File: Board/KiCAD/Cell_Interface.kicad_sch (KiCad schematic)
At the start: 32 parts, among them Q23 2N7002, Q24 2N7002, Q25 2N7002, Q26 2N7002, Q27 IRF9540NSTRLPBF, Q28 IRF9540NSTRLPBF, Q29 IRF9540NSTRLPBF, Q30 IRF9540NSTRLPBF, Q31 IRF9540NSTRLPBF, Q32 2N7002, Q33 IRF9540NSTRLPBF, U4 INA260, U6 INA260, U7 INA260, U8 INA260

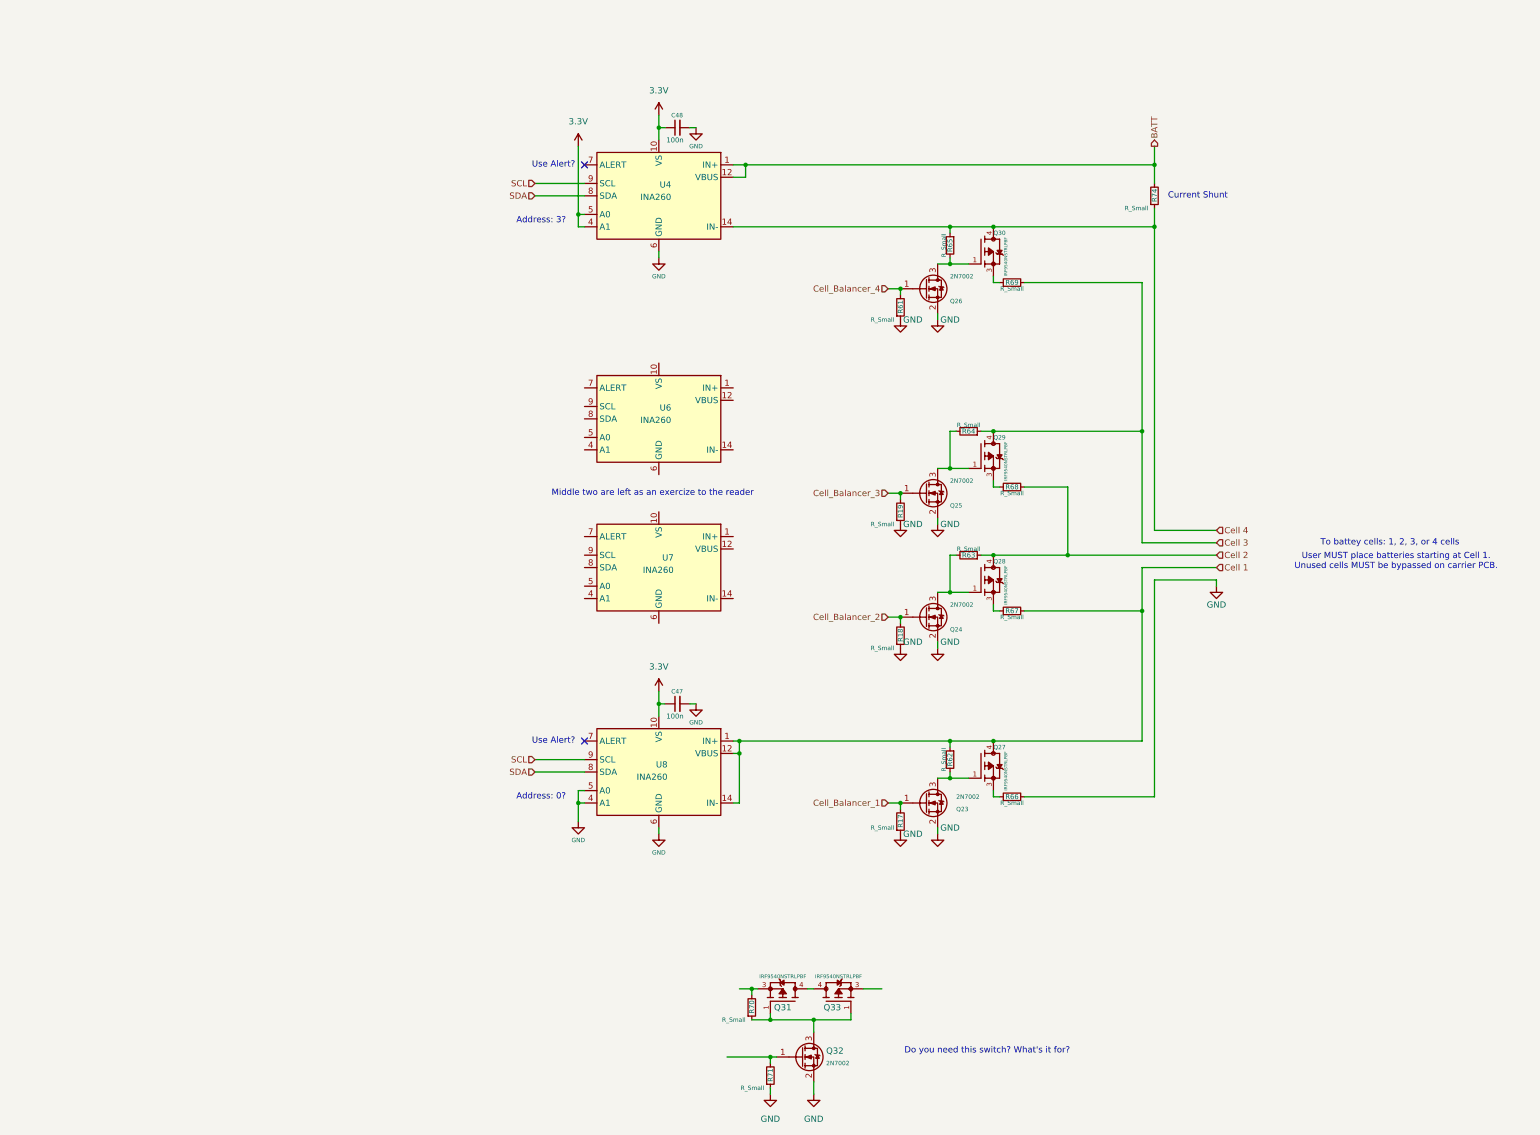
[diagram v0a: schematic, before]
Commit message: Add files via upload
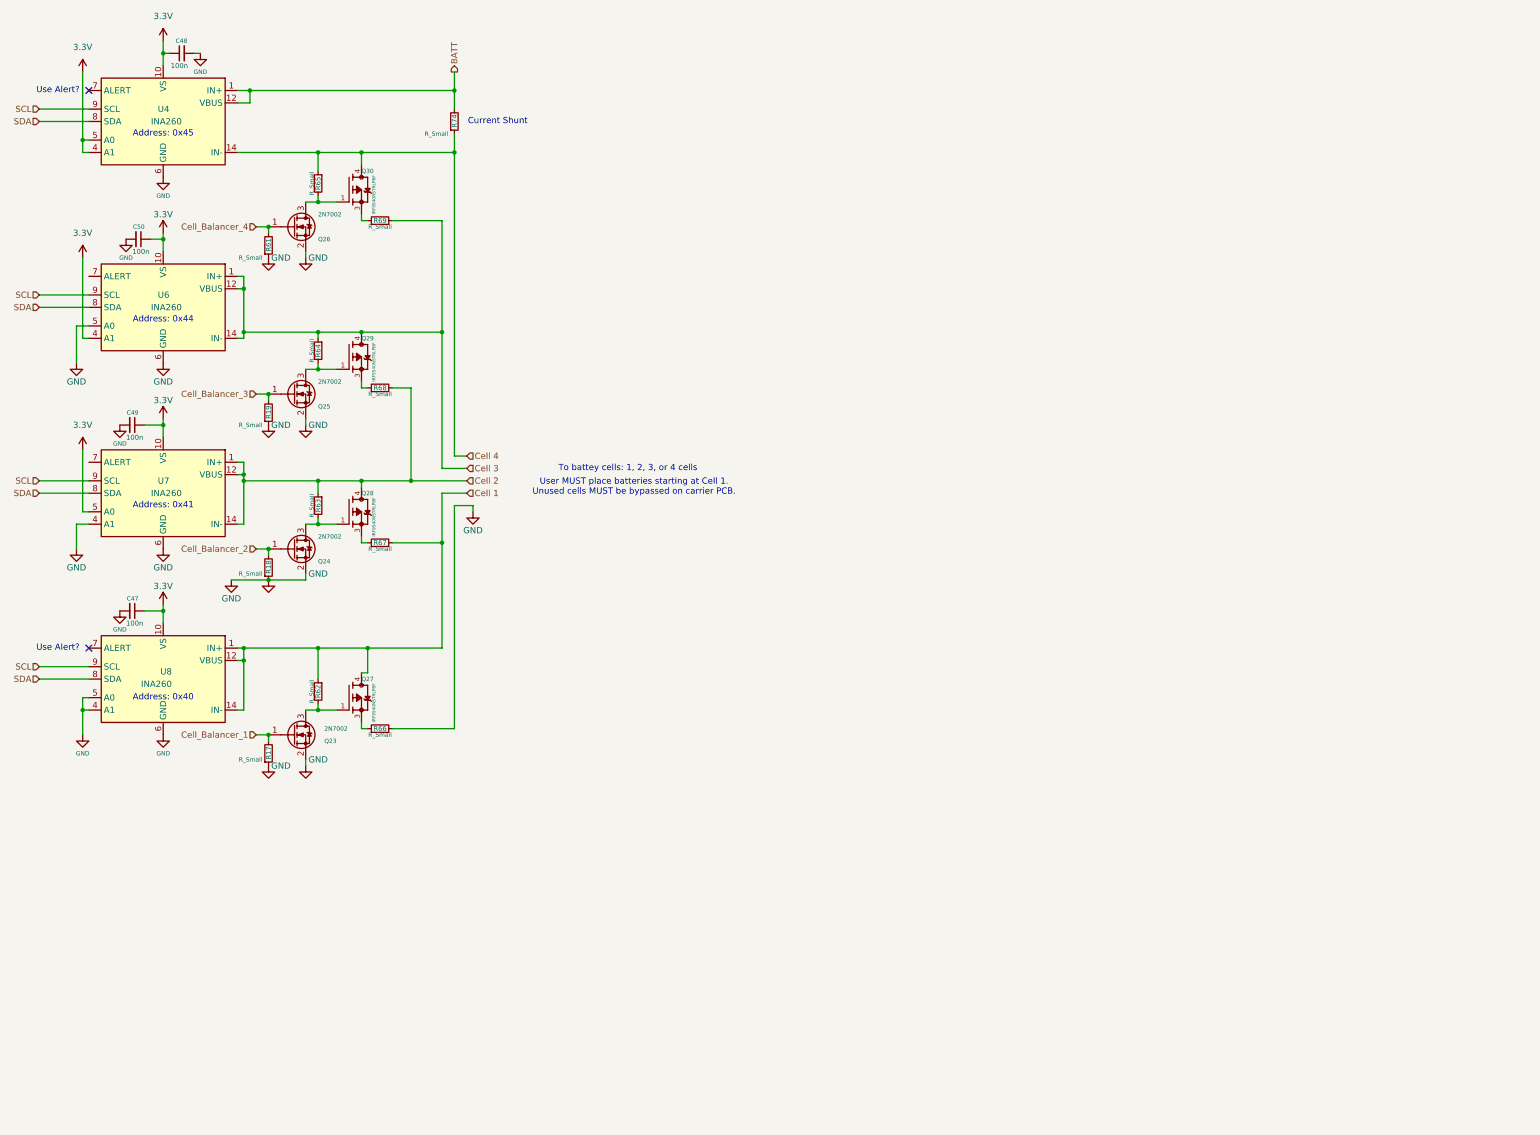
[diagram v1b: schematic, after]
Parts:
- removed Q31, Q33: IRF9540NSTRLPBF, IRF9540NSTRLPBF:DPAK254P1524X483-4_3N, symbol IRF9540NSTRLPBF:IRF9540NSTRLPBF
- removed Q32: 2N7002, Package_TO_SOT_SMD:SOT-23, symbol Transistor_FET:2N7002
- removed R70: R_Small, symbol Device:R_Small
- removed R71: R_Small, Resistor_SMD:R_0201_0603Metric, symbol Device:R_Small
- added C49, C50: 100n, Capacitor_SMD:C_0201_0603Metric, symbol Device:C_Small
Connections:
- net 3.3V: now also U6.10 (VS), U6.4 (A1), U7.10 (VS), U7.5 (A0), C49.1, C50.1
- net Cell 2: now also U7.1 (IN+), U7.12 (VBUS), U7.14 (IN-)
- net Cell 3: now also U6.1 (IN+), U6.12 (VBUS), U6.14 (IN-)
- net GND: now also U6.5 (A0), U6.6 (GND), U7.4 (A1), U7.6 (GND), C49.2, C50.2
- net SCL: now also U6.9 (SCL), U7.9 (SCL)
- net SDA: now also U6.8 (SDA), U7.8 (SDA)
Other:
- note added: "Address: 0x40"
- note added: "Address: 0x41"
- note added: "Address: 0x44"
- note added: "Address: 0x45"
- note removed: "Address: 0?"
- note removed: "Address: 3?"
- note removed: "Do you need this switch? What's it for?"
- note removed: "Middle two are left as an exercize to the reader"
- moved on the sheet: C47, C48, Q23, Q24, Q25, Q26, Q27, Q28, Q29, Q30, R17, R18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

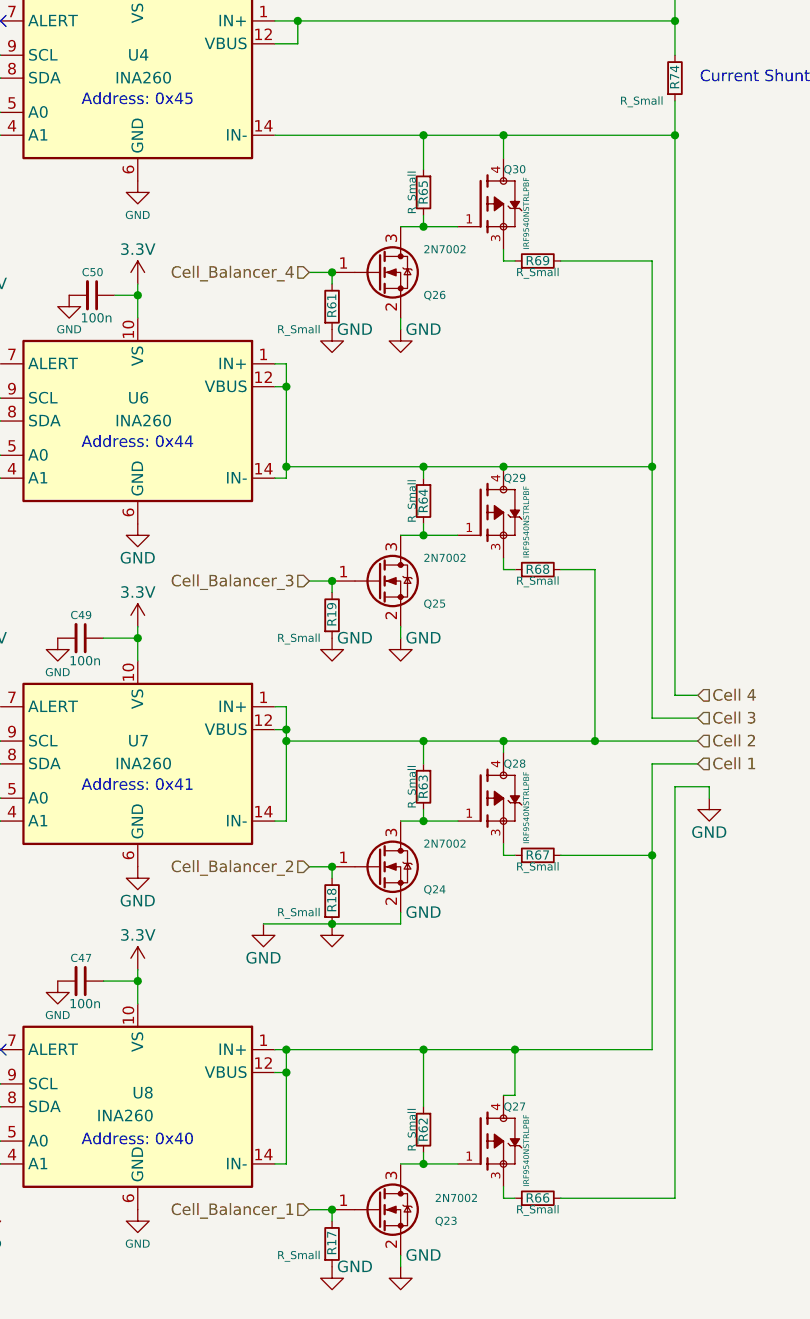
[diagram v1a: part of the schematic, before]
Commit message: Add files via upload
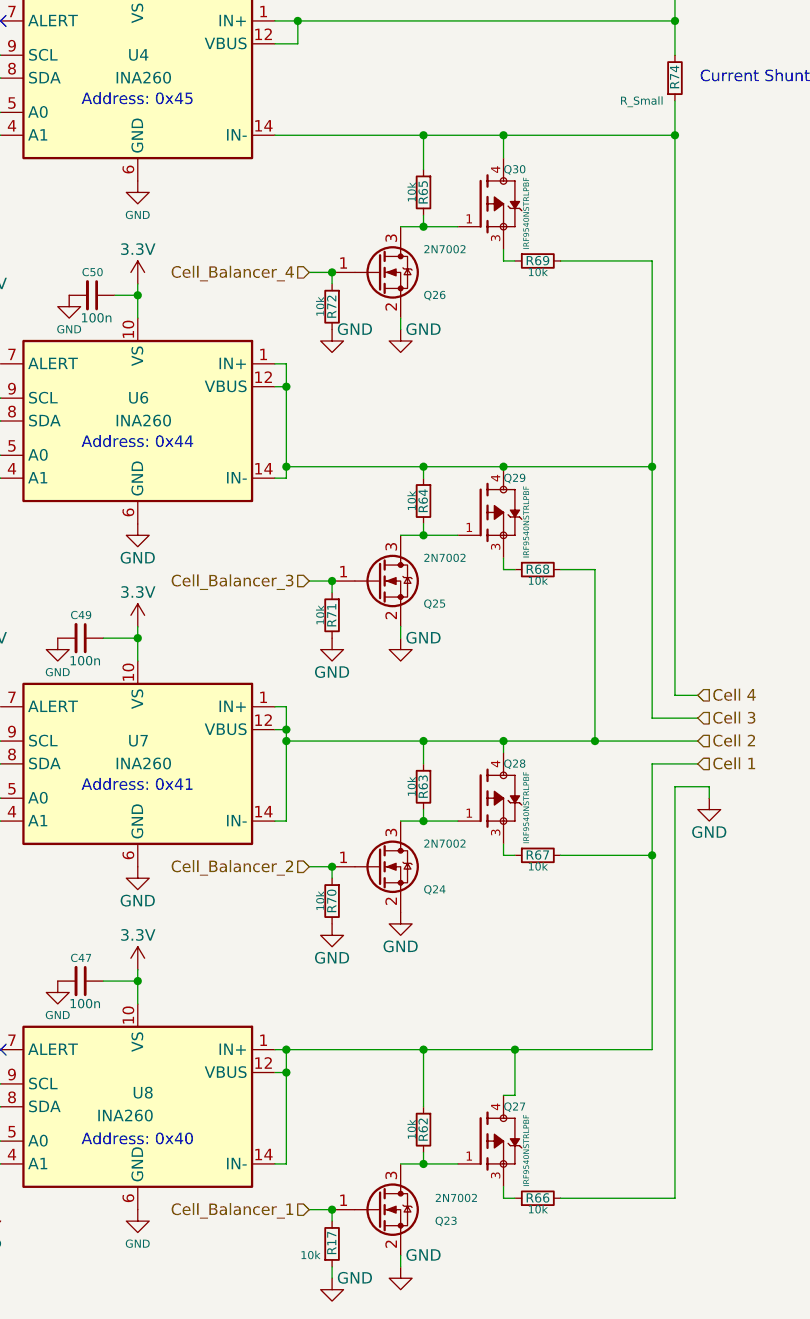
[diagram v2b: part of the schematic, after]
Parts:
- removed R18, R19, R61: R_Small, Resistor_SMD:R_0201_0603Metric, symbol Device:R_Small
- added R70, R71, R72: 10k, Resistor_SMD:R_0201_0603Metric, symbol Device:R_Small
- R17: value R_Small -> 10k
- R62, R63, R64, R65, R66, R67, R68, R69: value R_Small -> 10k; footprint (none) -> Resistor_SMD:R_0201_0603Metric
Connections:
- net Cell_Balancer_2: now also R70.1
- net Cell_Balancer_3: now also R71.1
- net Cell_Balancer_4: now also R72.1
- net GND: now also R70.2, R71.2, R72.2

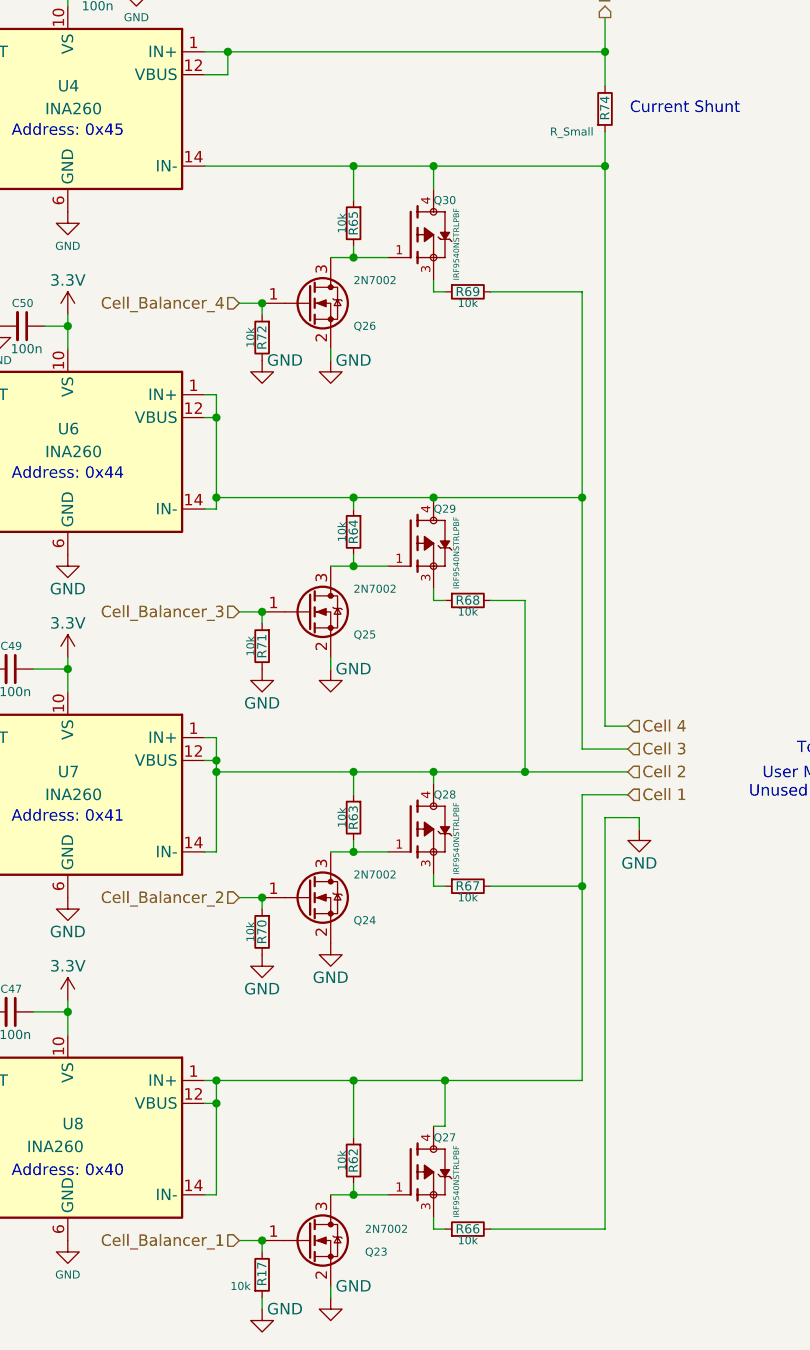
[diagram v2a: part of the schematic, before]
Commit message: Add files via upload
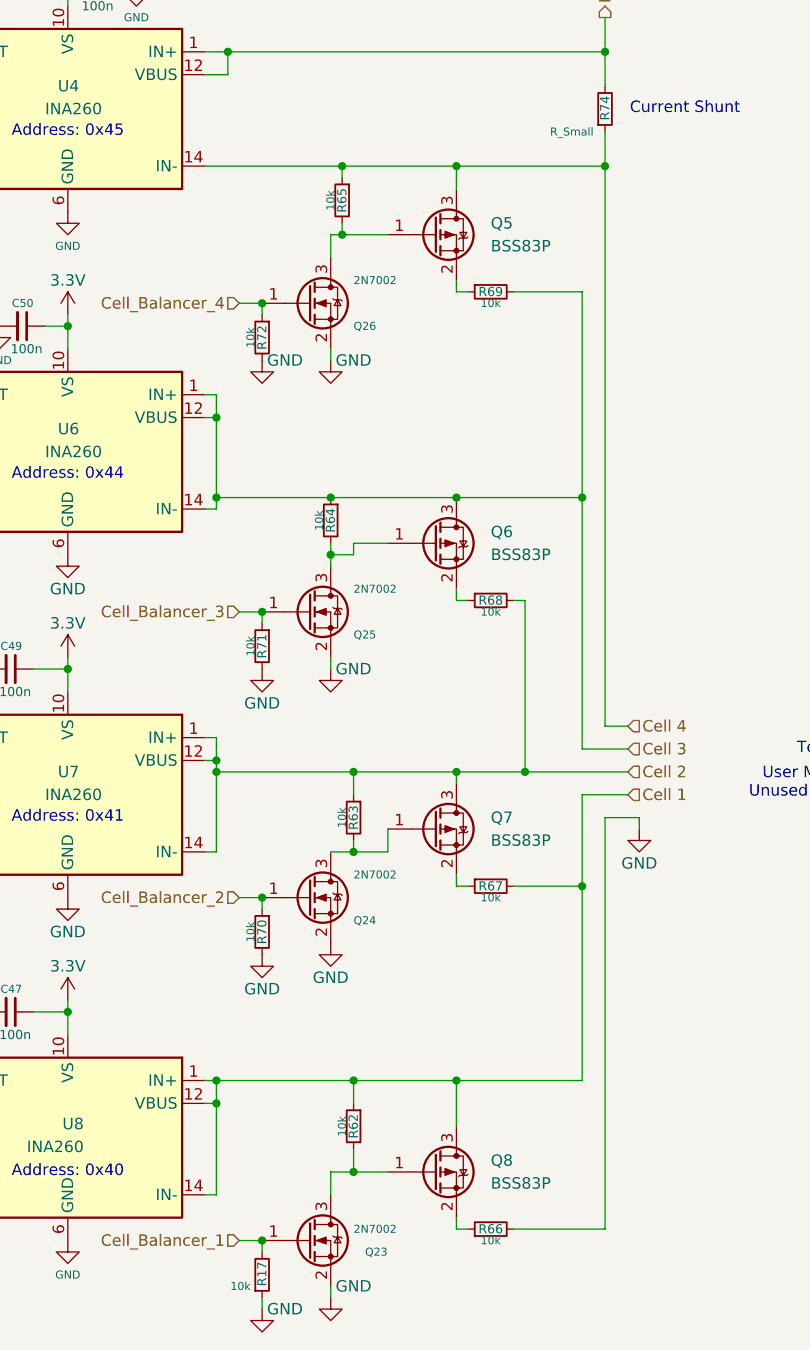
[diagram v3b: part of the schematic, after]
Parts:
- removed Q27, Q28, Q29, Q30: IRF9540NSTRLPBF, IRF9540NSTRLPBF:DPAK254P1524X483-4_3N, symbol IRF9540NSTRLPBF:IRF9540NSTRLPBF
- added Q5, Q6, Q7, Q8: BSS83P, Package_TO_SOT_SMD:SOT-23, symbol Transistor_FET:BSS83P
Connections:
- net Cell 1: now also Q8.3 (D)
- net Cell 2: now also Q7.3 (D)
- net Cell 3: now also Q6.3 (D)
- net Cell 4: now also Q5.3 (D)
- net at Q25.3 (D), R64.2: now also Q6.1 (G)
- net at R68.1: now also Q6.2 (S)
- net at Q23.3 (D), R62.2: now also Q8.1 (G)
- net at R66.1: now also Q8.2 (S)
- net at Q24.3 (D), R63.2: now also Q7.1 (G)
- net at Q26.3 (D), R65.2: now also Q5.1 (G)
- net at R67.1: now also Q7.2 (S)
- net at R69.1: now also Q5.2 (S)
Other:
- moved on the sheet: R62, R64, R65, R66, R67, R68, R69
